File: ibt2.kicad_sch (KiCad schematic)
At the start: 21 parts, among them J1 SIGNAL, J2 BATTERY, J3 MOTOR, Q1 BTN8982TA, Q2 BTN8982TA, U1 SN74HC244DW

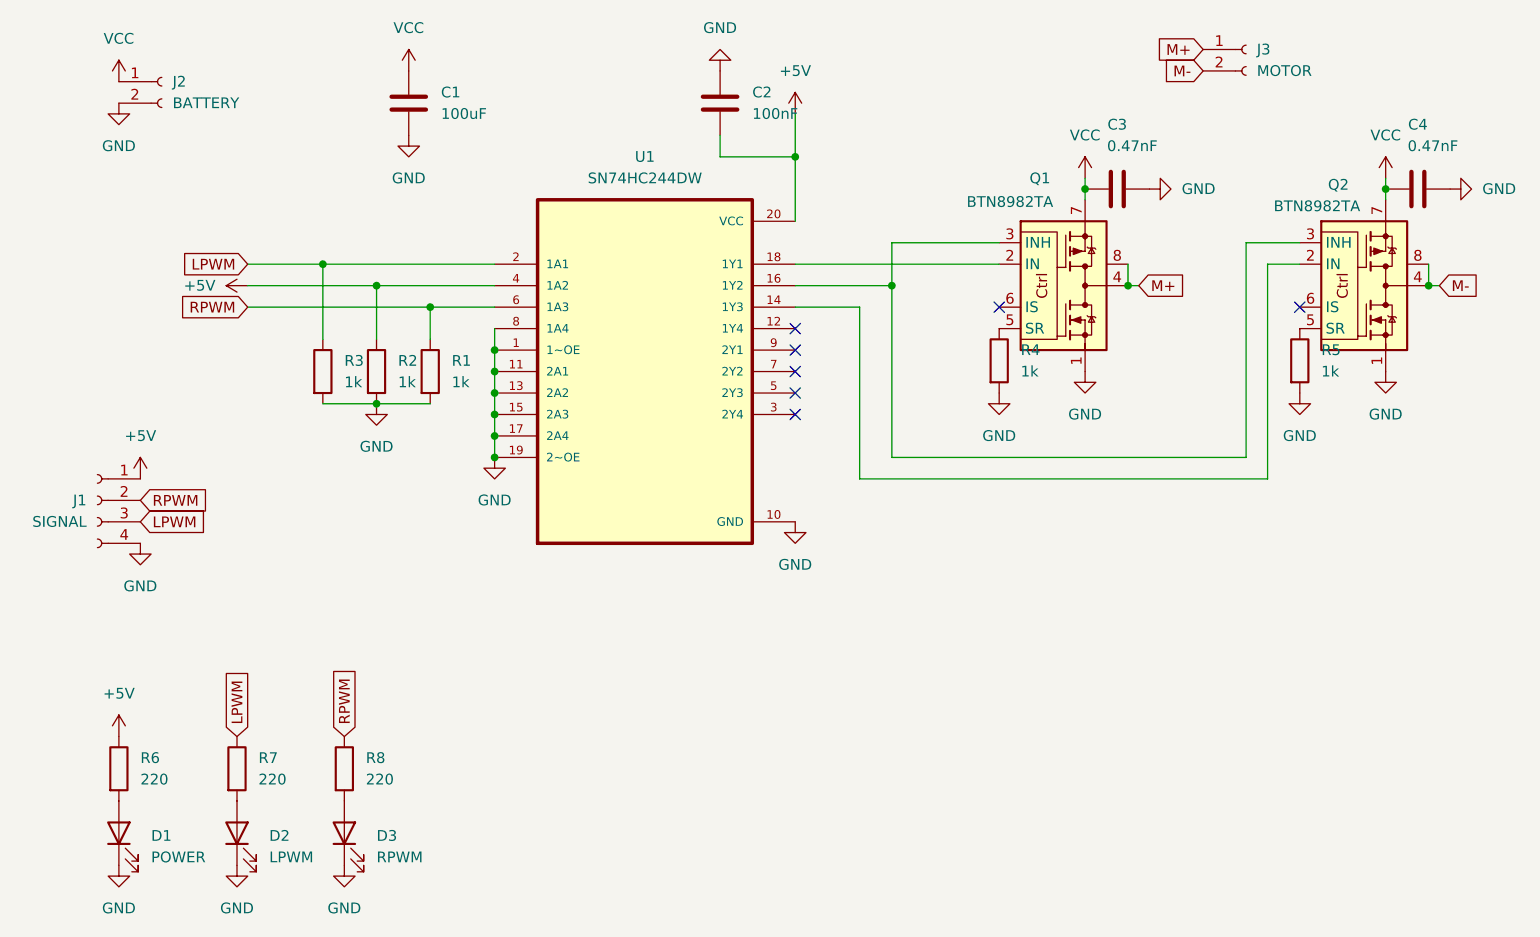
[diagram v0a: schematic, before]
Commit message: ..
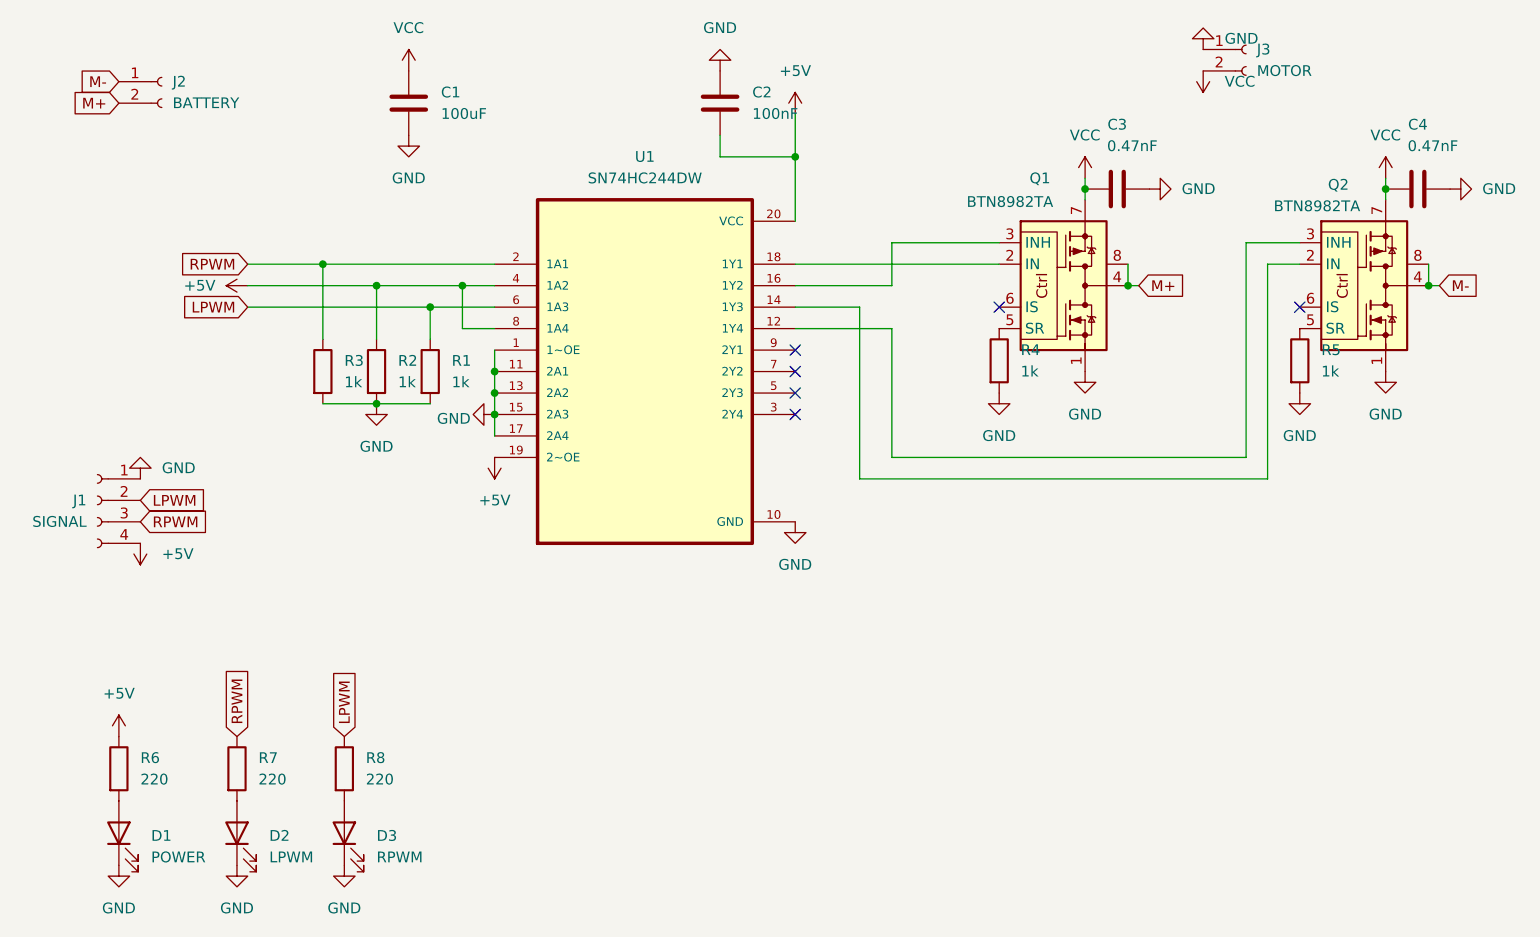
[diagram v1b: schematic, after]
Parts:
- D1, D2, D3: footprint LED_THT:LED_D5.0mm -> LED_THT:LED_D3.0mm
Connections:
- net +5V: now also J1.4 (Pin_4), U1.19 (2~OE), U1.8 (1A4); no longer J1.1 (Pin_1)
- net GND: now also J1.1 (Pin_1), J3.1 (Pin_1); no longer J1.4 (Pin_4), J2.2 (Pin_2), U1.19 (2~OE), U1.8 (1A4)
- net LPWM: now also J1.2 (Pin_2), R1.1, R8.1, U1.6 (1A3); no longer J1.3 (Pin_3), R3.1, R7.1, U1.2 (1A1)
- net M+: now also J2.2 (Pin_2); no longer J3.1 (Pin_1)
- net M-: now also J2.1 (Pin_1); no longer J3.2 (Pin_2)
- net RPWM: now also J1.3 (Pin_3), R3.1, R7.1, U1.2 (1A1); no longer J1.2 (Pin_2), R1.1, R8.1, U1.6 (1A3)
- net VCC: now also J3.2 (Pin_2); no longer J2.1 (Pin_1)
- net at Q1.3 (INH), U1.16 (1Y2): no longer Q2.3 (INH)
- net at U1.12 (1Y4): now also Q2.3 (INH)
- no-connect marks 7 -> 6

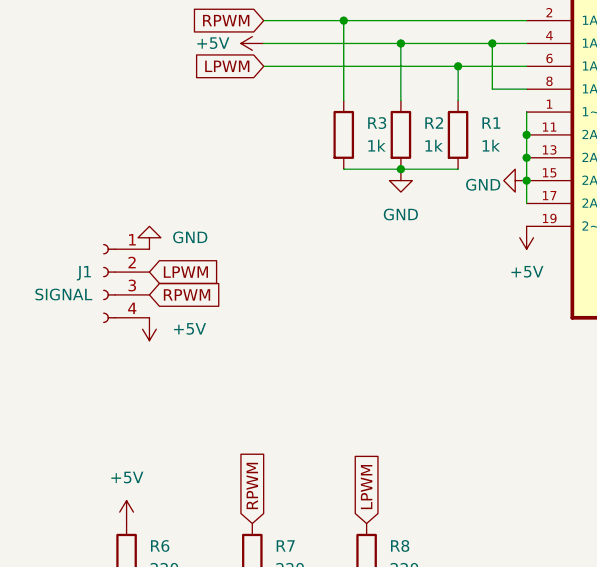
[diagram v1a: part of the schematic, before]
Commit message: ...
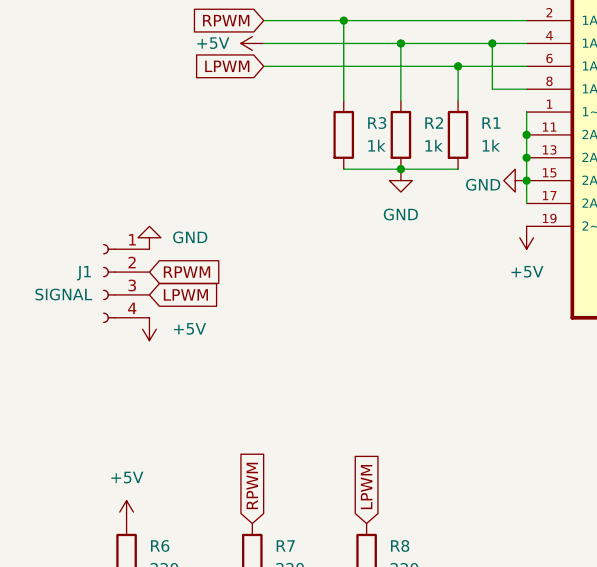
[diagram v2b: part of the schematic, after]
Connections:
- net LPWM: now also J1.3 (Pin_3); no longer J1.2 (Pin_2)
- net RPWM: now also J1.2 (Pin_2); no longer J1.3 (Pin_3)
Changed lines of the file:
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@@
-	(global_label "RPWM"
-		(shape input)
-		(at 34.29 76.2 0)
-		(fields_autoplaced yes)
-		(effects
-			(font
-				(size 1.27 1.27)
-			)
-			(justify left)
-		)
-		(property "Intersheetrefs" "${INTERSHEET_REFS}"
-			(at 42.718 76.2 0)
-			(effects
-				(font
-					(size 1.27 1.27)
-				)
-				(justify left)
-				(hide yes)
-			)
-		)
-	)
 	(global_label "RPWM"
 		(shape input)
@@
 	(global_label "LPWM"
 		(shape input)
+		(at 34.29 76.2 0)
+		(fields_autoplaced yes)
+		(effects
+			(font
+				(size 1.27 1.27)
+			)
+			(justify left)
+		)
+		(property "Intersheetrefs" "${INTERSHEET_REFS}"
+			(at 42.4761 76.2 0)
+			(effects
+				(font
+					(size 1.27 1.27)
+				)
+				(justify left)
+				(hide yes)
+			)
+		)
+	)
+	(global_label "RPWM"
+		(shape input)
 		(at 34.29 73.66 0)
 		(fields_autoplaced yes)
@@
 		)
 		(property "Intersheetrefs" "${INTERSHEET_REFS}"
-			(at 42.4761 73.66 0)
+			(at 42.718 73.66 0)
 			(effects
 				(font
